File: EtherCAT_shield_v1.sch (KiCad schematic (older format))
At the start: 3 parts

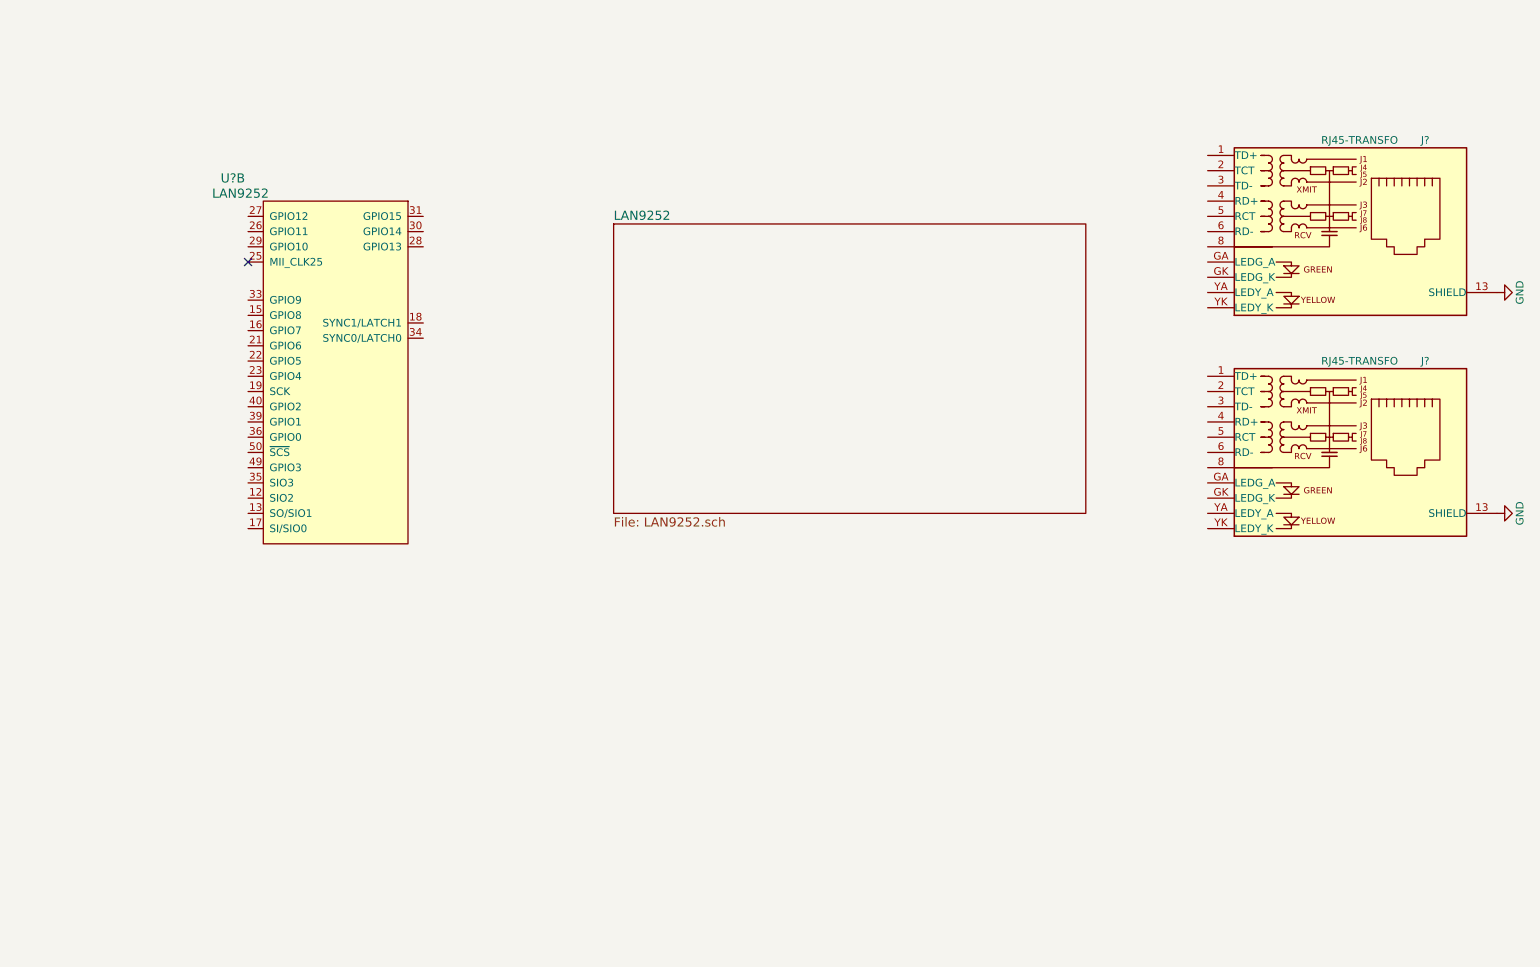
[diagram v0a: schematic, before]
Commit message: 配線
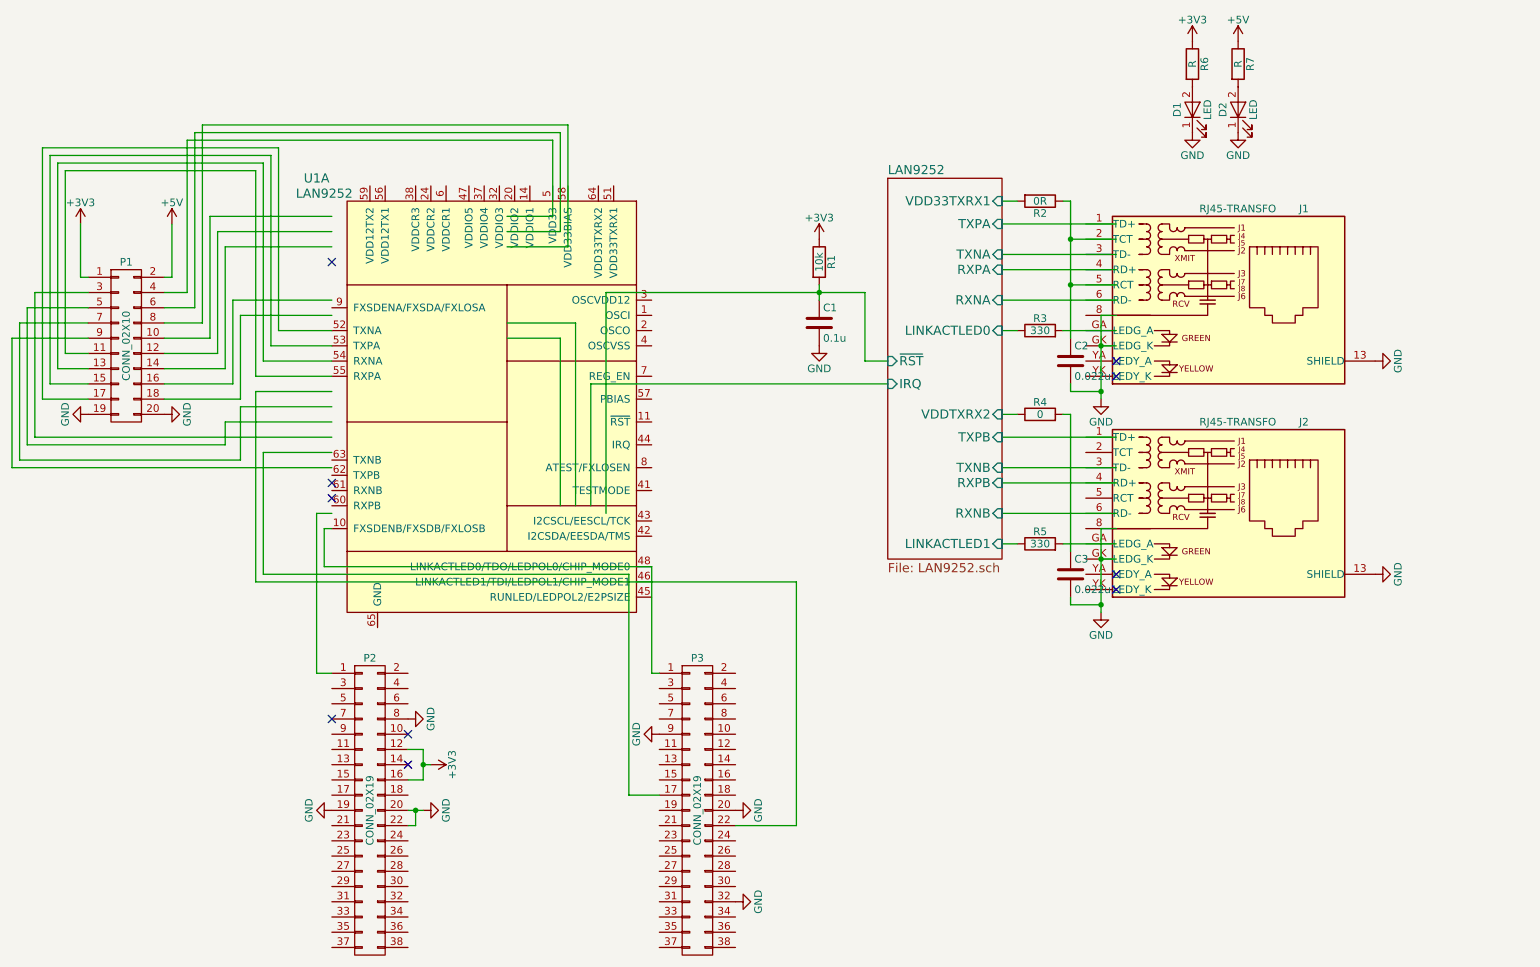
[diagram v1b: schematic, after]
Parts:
- added C1: 0.1u, symbol C
- added C2, C3: 0.022u, symbol C
- added D1, D2: LED, symbol LED
- added P1: CONN_02X10, symbol CONN_02X10
- added P2, P3: CONN_02X19, symbol CONN_02X19
- added R1: 10k, symbol R
- added R2: 0R, symbol R
- added R3, R5: 330, symbol R
- added R4: 0, symbol R
- added R6, R7: R, symbol R
- gave numbers to parts that had none: 3
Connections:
- net labels added: +3V3, +5V
- wire segments 0 -> 146
- no-connect marks 1 -> 10
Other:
- moved on the sheet: J1, J2
